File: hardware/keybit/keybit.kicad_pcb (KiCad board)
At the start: 2 copper layers, 19 x 19 mm, 23 parts, among them SW1 SW_Push, U1 CH32V003FxUx, U2 YZ13515055F-02025-02, U3 YZ13515055F-02025-02, U4 YZ13515055F-02025-02, U5 YZ13515055F-02025-02, U6 YZ13515055F-02025-02, U7 YZ13515055F-02025-02, U8 YZ13515055F-02025-02, U9 YZ13515055F-02025-02

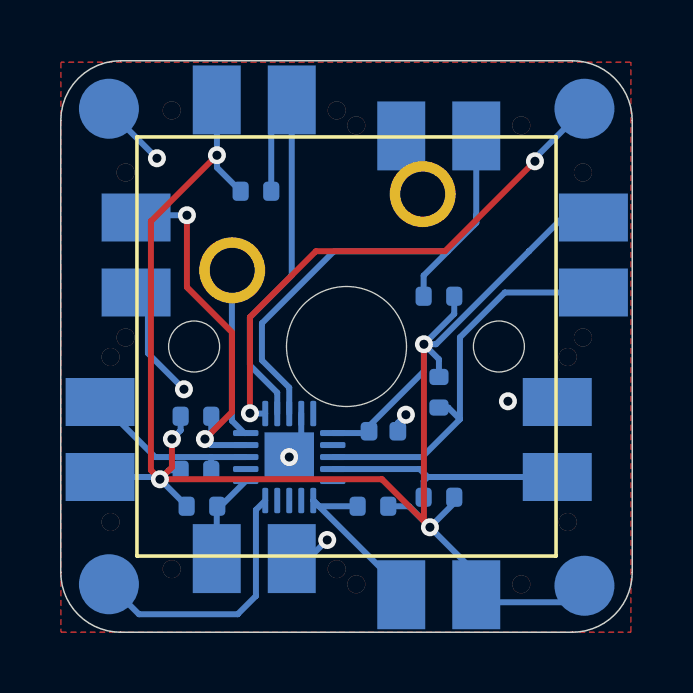
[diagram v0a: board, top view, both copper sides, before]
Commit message: blender and stuff
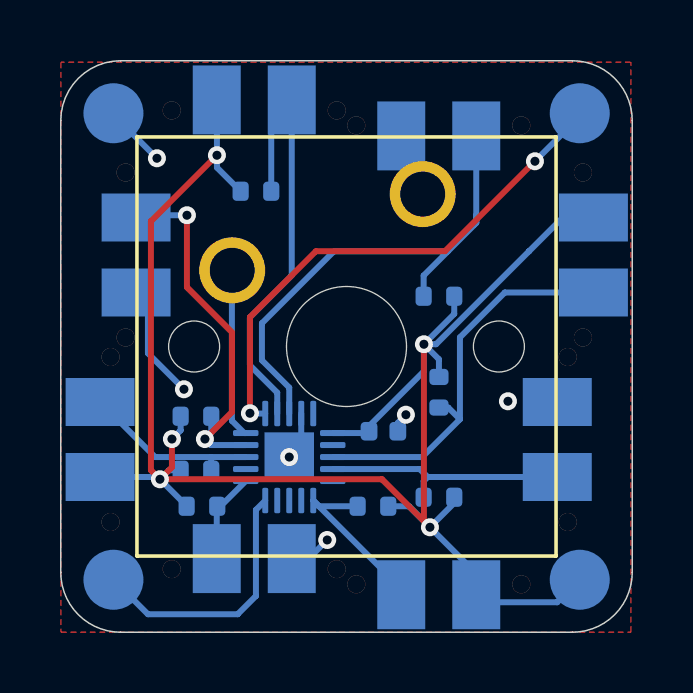
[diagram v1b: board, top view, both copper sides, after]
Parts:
- moved TP1 0.25 mm to (157.8, 84.0)
- moved TP3 0.22 mm to (157.8, 68.4)
- moved TP4 0.21 mm to (142.2, 68.4)
- moved TP2 0.21 mm to (142.2, 84.0)
